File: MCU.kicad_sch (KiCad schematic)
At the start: 14 parts, among them J3 Conn_02x03_Odd_Even, T2 TestPoint, U1 HDC2080, U3 ESP32-C6-MINI-1

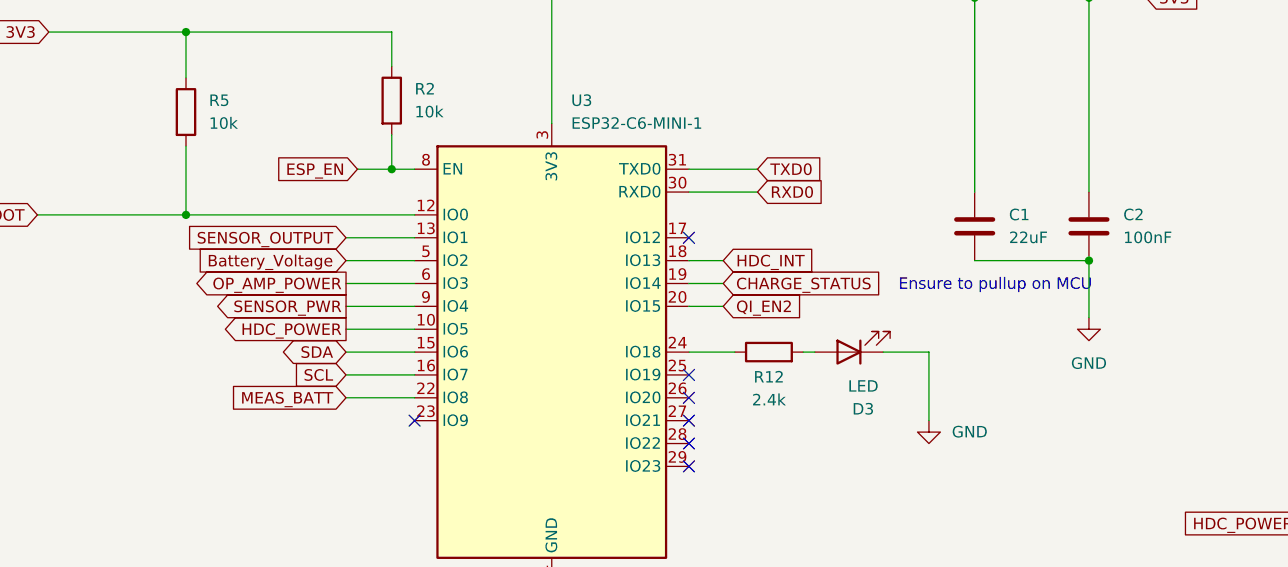
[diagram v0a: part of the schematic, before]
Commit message: laid out pcb
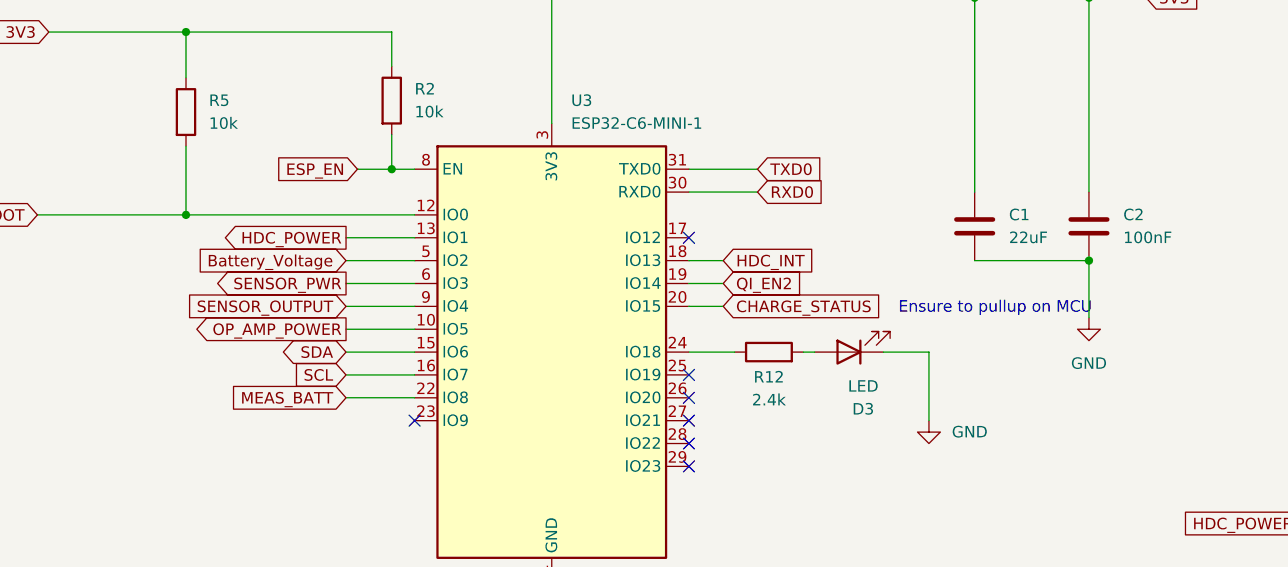
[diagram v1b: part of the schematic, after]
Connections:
- net CHARGE_STATUS: now also U3.20 (IO15); no longer U3.19 (IO14)
- net HDC_POWER: now also U3.13 (IO1); no longer U3.10 (IO5)
- net OP_AMP_POWER: now also U3.10 (IO5); no longer U3.6 (IO3)
- net QI_EN2: now also U3.19 (IO14); no longer U3.20 (IO15)
- net SENSOR_OUTPUT: now also U3.9 (IO4); no longer U3.13 (IO1)
- net SENSOR_PWR: now also U3.6 (IO3); no longer U3.9 (IO4)
